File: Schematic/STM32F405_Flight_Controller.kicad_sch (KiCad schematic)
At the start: 74 parts, among them J1 USB_C_Receptacle_USB2.0_16P, J2 XT60 (BATT), J3 ESC_1, J4 ESC_2, J5 ESC_3, J6 ESC_4, J7 SWD, SW1 SW_SPDT, SW2 SW_Push, U1 STM32F405RGTx, U4 AP7361C-33E, U5 LIS3MDL, U7 LMR33640DDDA, U8 W25Q128JVS, Y1 16MHz Crystal

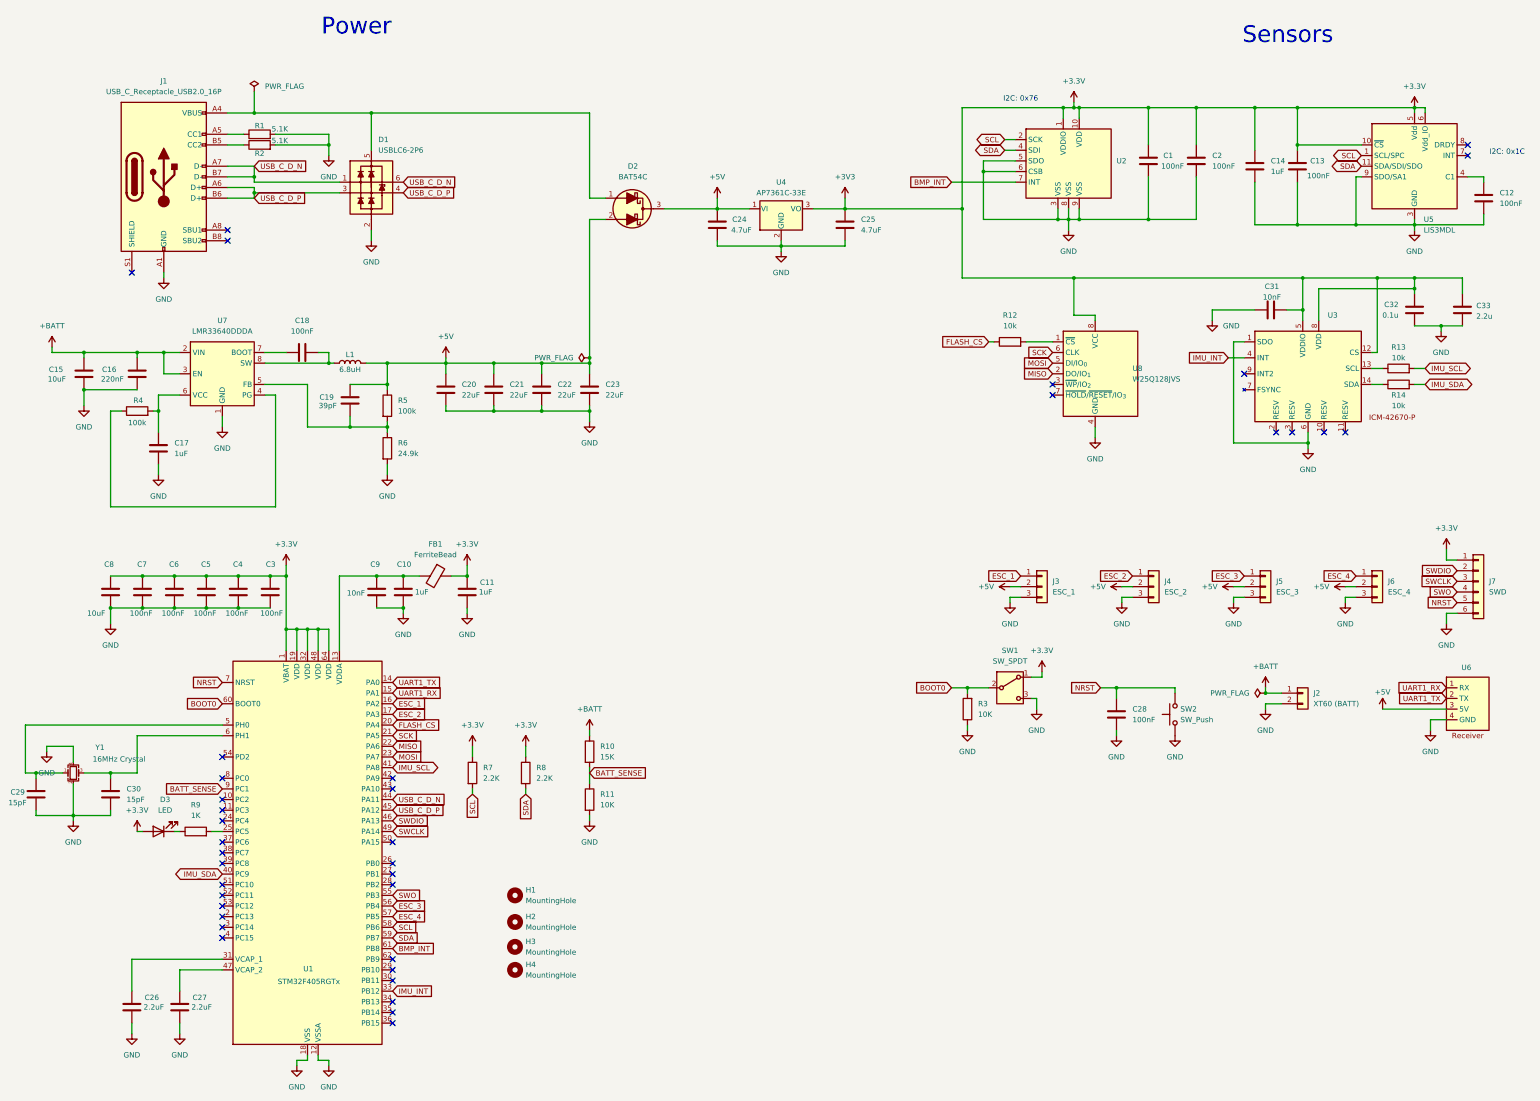
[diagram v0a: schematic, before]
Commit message: Add files via upload
Added sheets
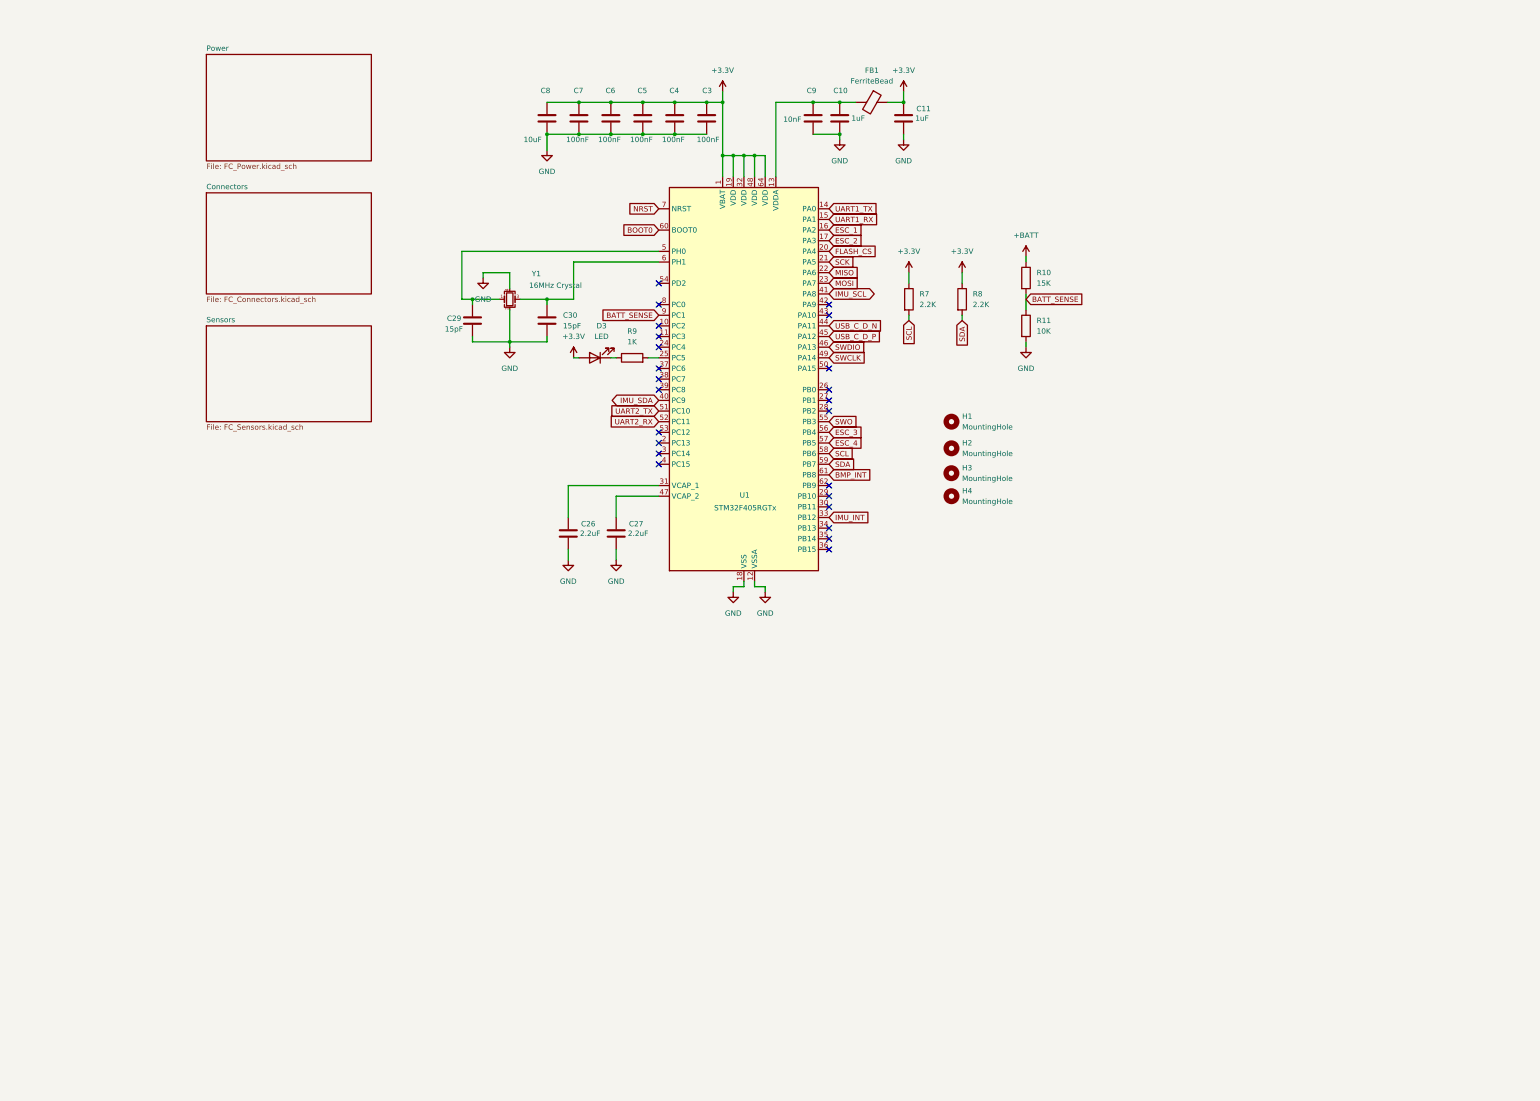
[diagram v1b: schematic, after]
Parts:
- removed C1, C18, C2, C28: 100nF, Capacitor_SMD:C_0603_1608Metric, symbol PCM_Capacitor_AKL:C_0402
- removed C12, C13: 100nF, Capacitor_SMD:C_0402_1005Metric, symbol PCM_Capacitor_AKL:C_0402
- removed C14: 1uF, Capacitor_SMD:C_0402_1005Metric, symbol PCM_Capacitor_AKL:C_0402
- removed C15: 10uF, Capacitor_SMD:C_0603_1608Metric, symbol PCM_Capacitor_AKL:C_0402
- removed C16: 220nF, Capacitor_SMD:C_0603_1608Metric, symbol PCM_Capacitor_AKL:C_0402
- removed C17: 1uF, Capacitor_SMD:C_0603_1608Metric, symbol PCM_Capacitor_AKL:C_0402
- removed C19: 39pF, Capacitor_SMD:C_0603_1608Metric, symbol PCM_Capacitor_AKL:C_0402
- removed C20, C21, C22, C23: 22uF, Capacitor_SMD:C_0603_1608Metric, symbol PCM_Capacitor_AKL:C_0402
- removed C24, C25: 4.7uF, Capacitor_SMD:C_0603_1608Metric, symbol PCM_Capacitor_AKL:C_0402
- removed C31: 10nF, Capacitor_SMD:C_0603_1608Metric, symbol PCM_Capacitor_AKL:C_0402
- removed C32: 0.1u, Capacitor_SMD:C_0603_1608Metric, symbol Device:C
- removed C33: 2.2u, Capacitor_SMD:C_0603_1608Metric, symbol Device:C
- removed D1: USBLC6-2P6, Package_TO_SOT_SMD:SOT-666, symbol PCM_Diode_TVS_AKL:USBLC6-2P6
- removed D2: BAT54C, Package_TO_SOT_SMD:SOT-23-3, symbol PCM_Diode_Schottky_AKL:BAT54C
- removed J1: USB_C_Receptacle_USB2.0_16P, Connector_USB:USB_C_Receptacle_HCTL_HC-TYPE-C-16P-01A, symbol Connector:USB_C_Receptacle_USB2.0_16P
- removed J2: XT60 (BATT), Connector_AMASS:AMASS_XT60-F_1x02_P7.20mm_Vertical, symbol Connector_Generic:Conn_01x02
- removed J3: ESC_1, Connector_PinSocket_2.54mm:PinSocket_1x03_P2.54mm_Vertical, symbol Connector_Generic:Conn_01x03
- removed J4: ESC_2, Connector_PinSocket_2.54mm:PinSocket_1x03_P2.54mm_Vertical, symbol Connector_Generic:Conn_01x03
- removed J5: ESC_3, Connector_PinSocket_2.54mm:PinSocket_1x03_P2.54mm_Vertical, symbol Connector_Generic:Conn_01x03
- removed J6: ESC_4, Connector_PinSocket_2.54mm:PinSocket_1x03_P2.54mm_Vertical, symbol Connector_Generic:Conn_01x03
- removed J7: SWD, Connector_PinHeader_2.54mm:PinHeader_1x06_P2.54mm_Vertical, symbol Connector_Generic:Conn_01x06
- removed L1: 6.8uH, Inductor_SMD:L_Vishay_IHLP-4040, symbol Device:L
- removed R1, R2: 5.1K, Resistor_SMD:R_0603_1608Metric, symbol Device:R
- removed R12, R13, R14: 10k, Resistor_SMD:R_0603_1608Metric, symbol Device:R
- removed R3: 10K, Resistor_SMD:R_0603_1608Metric, symbol Device:R
- removed R4, R5: 100k, Resistor_SMD:R_0603_1608Metric, symbol Device:R
- removed R6: 24.9k, Resistor_SMD:R_0603_1608Metric, symbol Device:R
- removed SW1: SW_SPDT, Button_Switch_SMD:SW_SPDT_PCM12, symbol Switch:SW_SPDT
- removed SW2: SW_Push, Button_Switch_THT:SW_PUSH_6mm_H4.3mm, symbol Switch:SW_Push
- removed U2: ~, Custom Footprints:BMP390L, symbol Custom_Symbols:ICM-42670
- removed U3: ~, Custom Footprints:XDCR_ICM-42670-P, symbol Custom_Symbols:ICM-42670-P
- removed U4: AP7361C-33E, Package_TO_SOT_SMD:SOT-223-3_TabPin2, symbol Regulator_Linear:AP7361C-33E
- removed U5: LIS3MDL, Package_LGA:LGA-12_2x2mm_P0.5mm, symbol Sensor_Magnetic:LIS3MDL
- removed U6: ~, Connector_PinHeader_2.54mm:PinHeader_1x04_P2.54mm_Vertical, symbol Custom_Symbols:ELRS_Nano_Receiver
- removed U7: LMR33640DDDA, Package_SO:Texas_HSOP-8-1EP_3.9x4.9mm_P1.27mm_ThermalVias, symbol Regulator_Switching:LMR33640DDDA
- removed U8: W25Q128JVS, Package_SO:SOIC-8_5.3x5.3mm_P1.27mm, symbol Memory_Flash:W25Q128JVS
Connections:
- net UART2_TX: now reaches U1.51 (PC10)
- net UART2_RX: now reaches U1.52 (PC11)
- no-connect marks 38 -> 24
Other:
- added sheet Connectors (FC_Connectors.kicad_sch)
- added sheet Power (FC_Power.kicad_sch)
- added sheet Sensors (FC_Sensors.kicad_sch)
- note removed: "I2C: 0x1C"
- note removed: "I2C: 0x76"
- note removed: "Power"
- note removed: "Sensors"
- moved on the sheet: C10, C11, C26, C27, C29, C3, C30, C4, C5, C6, C7, C8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
